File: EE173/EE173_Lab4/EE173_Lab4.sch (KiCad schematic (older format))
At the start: 33 parts

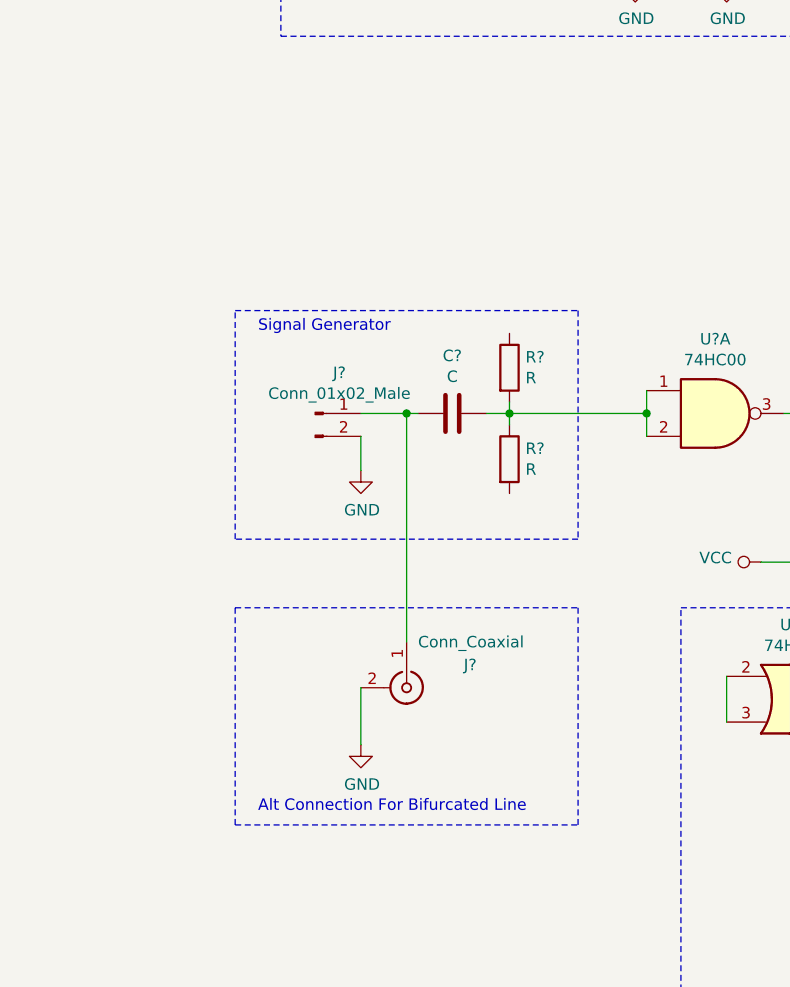
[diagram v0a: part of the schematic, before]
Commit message: The BNC connecter at the beginning was a huge mistake. The Bifurcated lines will be added from the other end (OSC connection in Lab 3). Instead I added a jumper at the source to choose between signal generator source or ground. Cleaned up a bit. Added jumper to short for source termination.
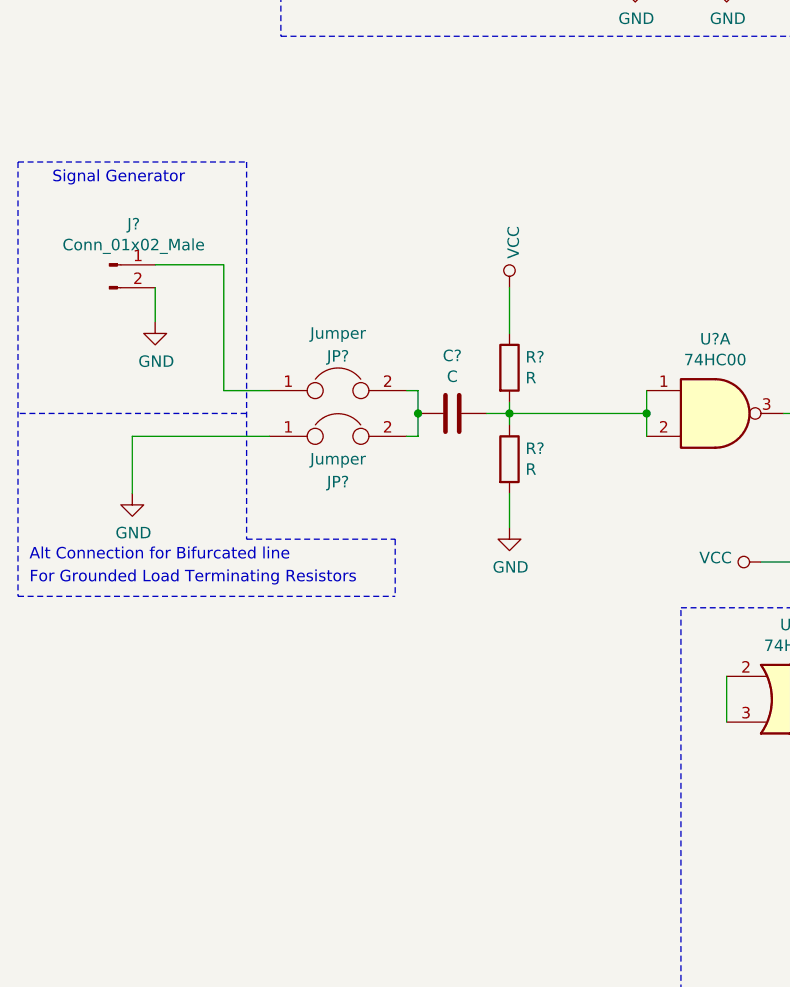
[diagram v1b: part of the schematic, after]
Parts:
- removed J?: Conn_Coaxial, symbol EE173_Lab4-rescue:Conn_Coaxial-My_Connector
- added JP? (x2): Jumper, symbol Device:Jumper
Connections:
- net GND: now also R?.2, JP?.1
- net VCC: now also R?.1
- net at J?.1 (Pin_1): now also JP?.1; no longer C?.2
- new net: C?.2, JP?.2, JP?.2
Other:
- note added: "Alt Connection for Bifurcated line"
- note added: "For Grounded Load Terminating Resistors"
- note removed: "Alt Connection For Bifurcated Line"
- moved on the sheet: J?
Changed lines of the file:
@@
 L Connector:Conn_01x02_Male J?
 U 1 1 5BF34C06
-P 3050 4300
-F 0 "J?" H 3156 4478 50  0000 C CNN
-F 1 "Conn_01x02_Male" H 3156 4387 50  0000 C CNN
-F 2 "" H 3050 4300 50  0001 C CNN
-F 3 "~" H 3050 4300 50  0001 C CNN
-	1    3050 4300
-	1    0    0    -1
-$EndComp
-$Comp
-L power:GND #PWR?
+P 2150 3650
+F 0 "J?" H 2256 3828 50  0000 C CNN
+F 1 "Conn_01x02_Male" H 2256 3737 50  0000 C CNN
+F 2 "" H 2150 3650 50  0001 C CNN
+F 3 "~" H 2150 3650 50  0001 C CNN
+	1    2150 3650
+	1    0    0    -1
+$EndComp
+$Comp
+L power:GND #PWR0101
 U 1 1 5BF34E41
-P 3250 4550
-F 0 "#PWR?" H 3250 4300 50  0001 C CNN
-F 1 "GND" H 3255 4377 50  0000 C CNN
-F 2 "" H 3250 4550 50  0001 C CNN
-F 3 "" H 3250 4550 50  0001 C CNN
-	1    3250 4550
+P 2350 3900
+F 0 "#PWR0101" H 2350 3650 50  0001 C CNN
+F 1 "GND" H 2355 3727 50  0000 C CNN
+F 2 "" H 2350 3900 50  0001 C CNN
+F 3 "" H 2350 3900 50  0001 C CNN
+	1    2350 3900
 	1    0    0    -1
 $EndComp
@@
 	0    1    1    0
 $EndComp
-Wire Wire Line
-	3250 4300 3450 4300
 $Comp
 L Device:R R?
@@
 Connection ~ 3900 4300
 $Comp
-L power:VCC #PWR?
+L power:VCC #PWR0102
 U 1 1 5BF3574A
 P 5000 4950
-F 0 "#PWR?" H 5000 4800 50  0001 C CNN
+F 0 "#PWR0102" H 5000 4800 50  0001 C CNN
 F 1 "VCC" V 5018 5077 50  0000 L CNN
 F 2 "" H 5000 4950 50  0001 C CNN
@@
 	8850 5050 8850 5100
 $Comp
-L power:GND #PWR?
+L power:GND #PWR0103
 U 1 1 5BF5C968
 P 9450 5350
-F 0 "#PWR?" H 9450 5100 50  0001 C CNN
+F 0 "#PWR0103" H 9450 5100 50  0001 C CNN
 F 1 "GND" H 9455 5177 50  0000 C CNN
 F 2 "" H 9450 5350 50  0001 C CNN
@@
 $EndComp
 $Comp
-L power:GND #PWR?
+L power:GND #PWR0104
 U 1 1 5BF5CE83
 P 9450 6050
-F 0 "#PWR?" H 9450 5800 50  0001 C CNN
+F 0 "#PWR0104" H 9450 5800 50  0001 C CNN
 F 1 "GND" H 9455 5877 50  0000 C CNN
 F 2 "" H 9450 6050 50  0001 C CNN
@@
 $EndComp
 $Comp
-L power:GND #PWR?
+L power:GND #PWR0105
 U 1 1 5BF62FC3
 P 5650 3850
-F 0 "#PWR?" H 5650 3600 50  0001 C CNN
+F 0 "#PWR0105" H 5650 3600 50  0001 C CNN
 F 1 "GND" H 5655 3677 50  0000 C CNN
 F 2 "" H 5650 3850 50  0001 C CNN
@@
 $EndComp
 $Comp
-L power:GND #PWR?
+L power:GND #PWR0106
 U 1 1 5BF643B0
 P 3900 2200
-F 0 "#PWR?" H 3900 1950 50  0001 C CNN
+F 0 "#PWR0106" H 3900 1950 50  0001 C CNN
 F 1 "GND" H 3905 2027 50  0000 C CNN
 F 2 "" H 3900 2200 50  0001 C CNN
@@
 $EndComp
 $Comp
-L power:GND #PWR?
+L power:GND #PWR0107
 U 1 1 5BF6476A
 P 6700 2050
-F 0 "#PWR?" H 6700 1800 50  0001 C CNN
+F 0 "#PWR0107" H 6700 1800 50  0001 C CNN
 F 1 "GND" H 6705 1877 50  0000 C CNN
 F 2 "" H 6700 2050 50  0001 C CNN
@@
 $EndComp
 $Comp
-L power:GND #PWR?
+L power:GND #PWR0108
 U 1 1 5BF64B24
 P 4850 2400
-F 0 "#PWR?" H 4850 2150 50  0001 C CNN
+F 0 "#PWR0108" H 4850 2150 50  0001 C CNN
 F 1 "GND" H 4855 2227 50  0000 C CNN
 F 2 "" H 4850 2400 50  0001 C CNN
@@
 $EndComp
 $Comp
-L power:GND #PWR?
+L power:GND #PWR0109
 U 1 1 5BF64EDE
 P 5250 2400
-F 0 "#PWR?" H 5250 2150 50  0001 C CNN
+F 0 "#PWR0109" H 5250 2150 50  0001 C CNN
 F 1 "GND" H 5255 2227 50  0000 C CNN
 F 2 "" H 5250 2400 50  0001 C CNN
@@
 $EndComp
 $Comp
-L power:VCC #PWR?
+L power:VCC #PWR0110
 U 1 1 5BF65AF9
 P 5250 1900
-F 0 "#PWR?" H 5250 1750 50  0001 C CNN
+F 0 "#PWR0110" H 5250 1750 50  0001 C CNN
 F 1 "VCC" H 5267 2073 50  0000 C CNN
 F 2 "" H 5250 1900 50  0001 C CNN
@@
 	4450 2000 4550 2000
 $Comp
-L power:GND #PWR?
+L power:GND #PWR0111
 U 1 1 5BF6AE55
 P 4450 2400
-F 0 "#PWR?" H 4450 2150 50  0001 C CNN
+F 0 "#PWR0111" H 4450 2150 50  0001 C CNN
 F 1 "GND" H 4455 2227 50  0000 C CNN
 F 2 "" H 4450 2400 50  0001 C CNN
@@
 Text Notes 3050 1700 0    50   ~ 0
 Power Supply
-Wire Notes Line
-	4200 3850 4200 4850
-Wire Notes Line
-	4200 4850 2700 4850
-Wire Notes Line
-	2700 4850 2700 3850
-Wire Notes Line
-	2700 3850 4200 3850
-Text Notes 2800 3950 0    50   ~ 0
+Text Notes 1900 3300 0    50   ~ 0
 Signal Generator
 $Comp
@@
 	6100 6300 6100 5750
 $Comp
-L power:GND #PWR?
+L power:GND #PWR0112
 U 1 1 5BFA5B7F
 P 5500 6650
-F 0 "#PWR?" H 5500 6400 50  0001 C CNN
+F 0 "#PWR0112" H 5500 6400 50  0001 C CNN
 F 1 "GND" H 5505 6477 50  0000 C CNN
 F 2 "" H 5500 6650 50  0001 C CNN
@@
 	7100 5650 7100 5750
 Wire Wire Line
-	3250 4400 3250 4550
-$Comp
-L power:GND #PWR?
+	2350 3750 2350 3900
+$Comp
+L power:GND #PWR0113
 U 1 1 5BFAAF3C
 P 6100 2800
-F 0 "#PWR?" H 6100 2550 50  0001 C CNN
+F 0 "#PWR0113" H 6100 2550 50  0001 C CNN
 F 1 "GND" H 6105 2627 50  0000 C CNN
 F 2 "" H 6100 2800 50  0001 C CNN
@@
 	8850 4650 8850 4450
 $Comp
-L EE173_Lab4-rescue:Conn_Coaxial-My_Connector J?
-U 1 1 5BFB3354
-P 3450 5500
-F 0 "J?" V 3350 5750 50  0000 L CNN
-F 1 "Conn_Coaxial" V 3250 5550 50  0000 L CNN
-F 2 "" H 3450 5500 50  0001 C CNN
-F 3 " ~" H 3450 5500 50  0001 C CNN
-	1    3450 5500
-	0    1    1    0
-$EndComp
+L Device:Jumper JP?
+U 1 1 5BFC95F1
+P 3150 4200
+F 0 "JP?" H 3150 4350 50  0000 C CNN
+F 1 "Jumper" H 3150 4450 50  0000 C CNN
+F 2 "" H 3150 4200 50  0001 C CNN
+F 3 "~" H 3150 4200 50  0001 C CNN
+	1    3150 4200
+	1    0    0    -1
+$EndComp
+$Comp
+L Device:Jumper JP?
+U 1 1 5BFCA8E8
+P 3150 4400
+F 0 "JP?" H 3150 4200 50  0000 C CNN
+F 1 "Jumper" H 3150 4300 50  0000 C CNN
+F 2 "" H 3150 4400 50  0001 C CNN
+F 3 "~" H 3150 4400 50  0001 C CNN
+	1    3150 4400
+	1    0    0    -1
+$EndComp
+Wire Wire Line
+	3500 4300 3500 4200
+Wire Wire Line
+	3500 4200 3450 4200
+Wire Wire Line
+	3500 4300 3500 4400
+Wire Wire Line
+	3500 4400 3450 4400
+Connection ~ 3500 4300
+$Comp
+L power:VCC #PWR?
+U 1 1 5BFCFBE7
+P 3900 3750
+F 0 "#PWR?" H 3900 3600 50  0001 C CNN
+F 1 "VCC" V 3918 3877 50  0000 L CNN
+F 2 "" H 3900 3750 50  0001 C CNN
+F 3 "" H 3900 3750 50  0001 C CNN
+	1    3900 3750
+	1    0    0    -1
+$EndComp
+Wire Wire Line
+	3900 3950 3900 3750
 $Comp
 L power:GND #PWR?
-U 1 1 5BFB335B
-P 3250 5750
-F 0 "#PWR?" H 3250 5500 50  0001 C CNN
-F 1 "GND" H 3255 5577 50  0000 C CNN
-F 2 "" H 3250 5750 50  0001 C CNN
-F 3 "" H 3250 5750 50  0001 C CNN
-	1    3250 5750
-	1    0    0    -1
-$EndComp
-Wire Wire Line
-	3250 5750 3250 5500
-Wire Wire Line
-	3450 5300 3450 4300
-Connection ~ 3450 4300
-Wire Wire Line
-	3450 4300 3500 4300
-Text Notes 2800 6050 0    50   ~ 0
-Alt Connection For Bifurcated Line
-Wire Notes Line
-	2700 5150 4200 5150
-Wire Notes Line
-	2700 6100 4200 6100
-Wire Notes Line
-	2700 5150 2700 6100
-Wire Notes Line
-	4200 5150 4200 6100
+U 1 1 5BFD3FF6
+P 3900 4800
+F 0 "#PWR?" H 3900 4550 50  0001 C CNN
+F 1 "GND" H 3905 4627 50  0000 C CNN
+F 2 "" H 3900 4800 50  0001 C CNN
+F 3 "" H 3900 4800 50  0001 C CNN
+	1    3900 4800
+	1    0    0    -1
+$EndComp
+Wire Wire Line
+	3900 4650 3900 4800
+Wire Wire Line
+	2350 3650 2650 3650
+Wire Wire Line
+	2650 3650 2650 4200
+Wire Wire Line
+	2650 4200 2850 4200
+$Comp
+L power:GND #PWR?
+U 1 1 5BFDA245
+P 2250 4650
+F 0 "#PWR?" H 2250 4400 50  0001 C CNN
+F 1 "GND" H 2255 4477 50  0000 C CNN
+F 2 "" H 2250 4650 50  0001 C CNN
+F 3 "" H 2250 4650 50  0001 C CNN
+	1    2250 4650
+	1    0    0    -1
+$EndComp
+Wire Wire Line
+	2250 4650 2250 4400
+Wire Wire Line
+	2250 4400 2850 4400
+Wire Notes Line
+	1750 3200 2750 3200
+Wire Notes Line
+	2750 4300 1750 4300
+Wire Notes Line
+	1750 3200 1750 5100
+Text Notes 1800 4950 0    50   ~ 0
+Alt Connection for Bifurcated line
+Text Notes 1800 5050 0    50   ~ 0
+For Grounded Load Terminating Resistors
+Wire Notes Line
+	2750 4850 3400 4850
+Wire Notes Line
+	3400 4850 3400 5100
+Wire Notes Line
+	1750 5100 3400 5100
+Wire Notes Line
+	2750 3200 2750 4850
 $EndSCHEMATC
